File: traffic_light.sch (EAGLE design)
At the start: 58 parts, among them IC1 74LS48N, IC2 74LS48N, IC3 NE555N, IC4 74LS48N, IC5 74LS48N, IC6 74190N, IC7 74190N

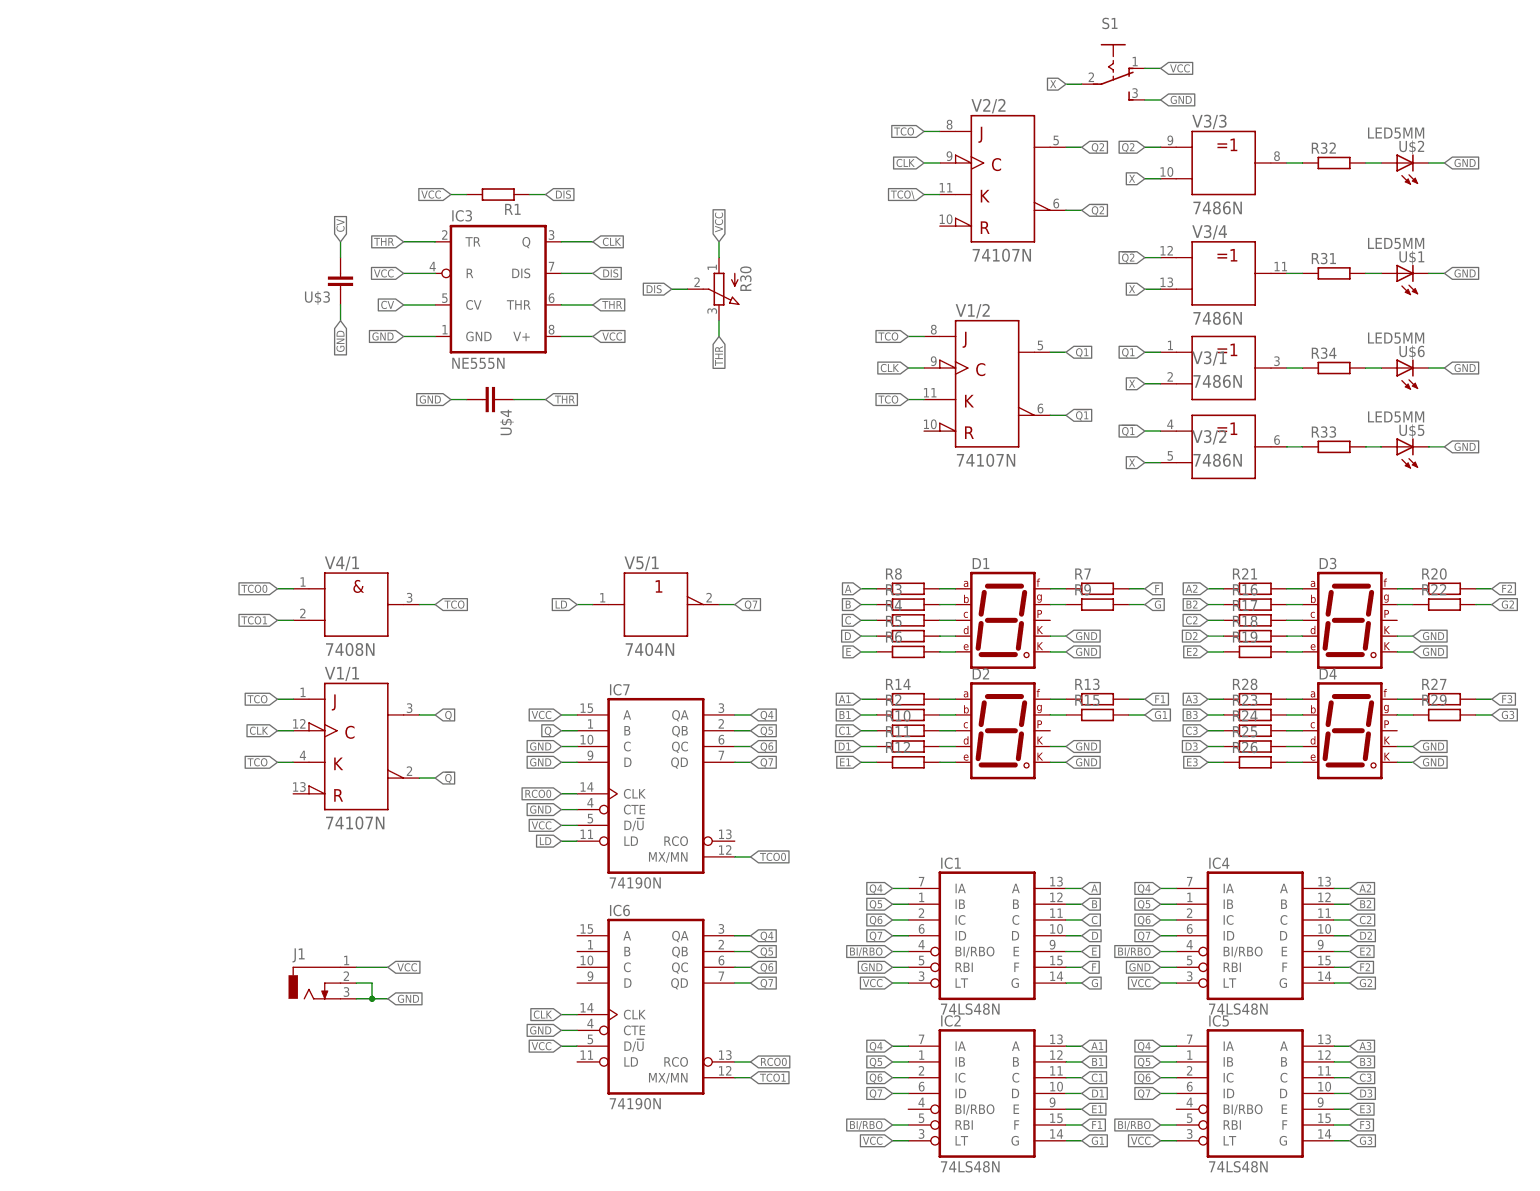
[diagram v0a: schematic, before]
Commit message: commit
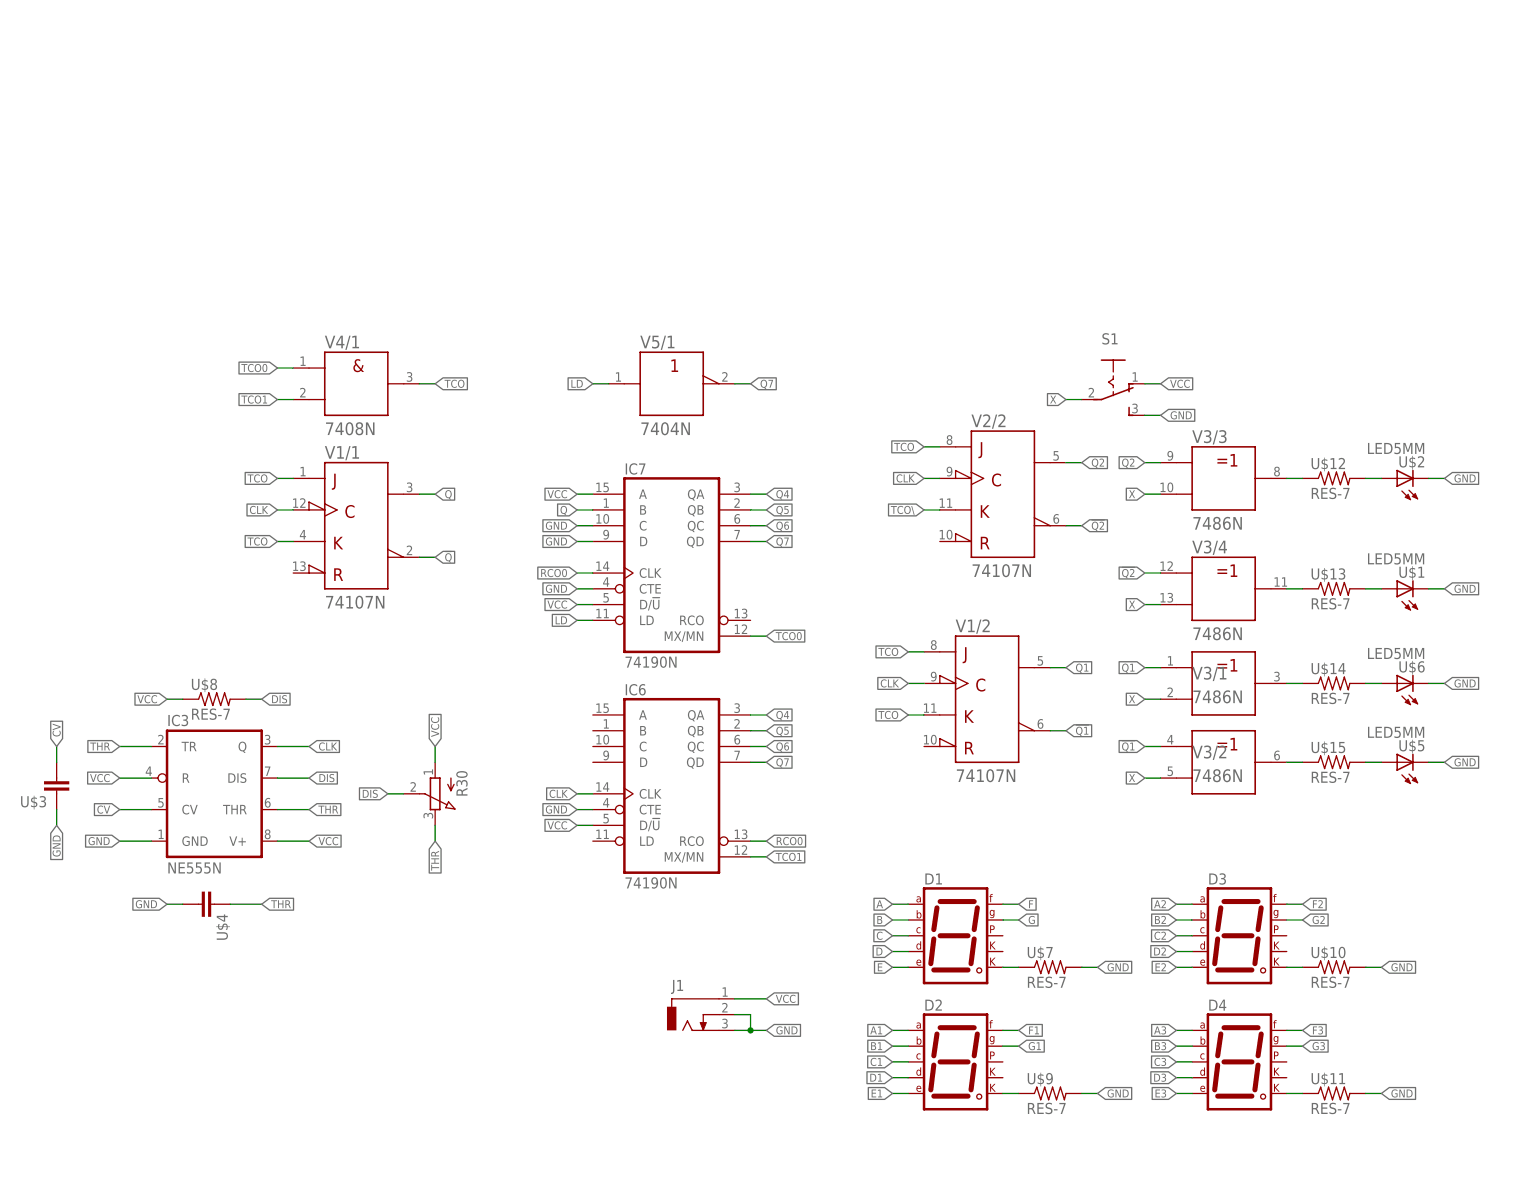
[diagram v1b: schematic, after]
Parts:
- removed IC1, IC2, IC4, IC5: 74LS48N, 74xx-eu:74LS48N
- removed R1, R10, R11, R12, R13, R14, R15, R16, R17, R18, R19, R2, R20, R21, R22, R23, R24, R25, R26, R27, R28, R29, R3, R31, R32, R33, R34, R4, R5, R6, R7, R8, R9: (no value), rcl:R-EU_0207/10
- added U$10, U$11, U$12, U$13, U$14, U$15, U$7, U$8, U$9: RES-7, MIA_LIBRARY-2-2-2:RES-7
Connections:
- removed net BI/RBO: IC1A.BI/RBO, IC2A.RBI, IC4A.BI/RBO, IC5A.RBI
- removed net N$10: D2.D, R11.2
- removed net N$11: D2.E, R12.2
- removed net N$12: D2.F, R13.1
- removed net N$13: D2.G, R15.1
- removed net N$14: D3.B, R16.2
- removed net N$15: D3.C, R17.2
- removed net N$16: D3.D, R18.2
- removed net N$17: D3.E, R19.2
- removed net N$18: D3.F, R20.1
- removed net N$19: D3.G, R22.1
- removed net N$20: D4.B, R23.2
- removed net N$21: D4.C, R24.2
- removed net N$22: D4.D, R25.2
- removed net N$23: D4.E, R26.2
- removed net N$24: D4.F, R27.1
- removed net N$25: D4.G, R29.1
- removed net N$5: D1.E, R6.2
- removed net N$6: D1.F, R7.1
- removed net N$7: D1.G, R9.1
- removed net N$8: D2.B, R2.2
- removed net N$9: D2.C, R10.2
- new net N$1: D1.CK2, U$7.1
- net A: no longer D2.A, D3.A, D4.A, IC1A.A, R14.2, R21.2, R28.2, R8.1, R8.2
- net A1: now also D2.A; no longer IC2A.A, R14.1
- net A2: now also D3.A; no longer IC4A.A, R21.1
- net A3: now also D4.A; no longer IC5A.A, R28.1
- net B: now also D1.B; no longer IC1A.B, R3.1
- net B1: now also D2.B; no longer IC2A.B, R2.1
- net B2: now also D3.B; no longer IC4A.B, R16.1
- net B3: now also D4.B; no longer IC5A.B, R23.1
- net C: now also D1.C; no longer IC1A.C, R4.1
- net C1: now also D2.C; no longer IC2A.C, R10.1
- net C2: now also D3.C; no longer IC4A.C, R17.1
- net C3: now also D4.C; no longer IC5A.C, R24.1
- net D: now also D1.D; no longer IC1A.D, R5.1
- net D1: now also D2.D; no longer IC2A.D, R11.1
- net D2: now also D3.D; no longer IC4A.D, R18.1
- net D3: now also D4.D; no longer IC5A.D, R25.1
- net DIS: now also U$8.2; no longer R1.1
- net E: now also D1.E; no longer IC1A.E, R6.1
- net E1: now also D2.E; no longer IC2A.E, R12.1
- net E2: now also D3.E; no longer IC4A.E, R19.1
- net E3: now also D4.E; no longer IC5A.E, R26.1
- net F: now also D1.F; no longer IC1A.F, R7.2
- net F1: now also D2.F; no longer IC2A.F, R13.2
- net F2: now also D3.F; no longer IC4A.F, R20.2
- net F3: now also D4.F; no longer IC5A.F, R27.2
- net G: now also D1.G; no longer IC1A.G, R9.2
- net G1: now also D2.G; no longer IC2A.G, R15.2
- net G2: now also D3.G; no longer IC4A.G, R22.2
- net G3: now also D4.G; no longer IC5A.G, R29.2
- net GND: now also U$10.2, U$11.2, U$7.2, U$9.2; no longer D1.CK1, D1.CK2, D2.CK1, D2.CK2, D3.CK1, D3.CK2, D4.CK1, D4.CK2, IC1A.RBI, IC4A.RBI
- net N$2: now also D2.CK2, U$9.1; no longer D1.B, R3.2
- net N$27: now also U$12.2; no longer R32.2
- net N$28: now also U$12.1; no longer R32.1
- net N$29: now also U$13.2; no longer R31.2
- net N$3: now also D3.CK2, U$10.1; no longer D1.C, R4.2
- net N$30: now also U$13.1; no longer R31.1
- net N$31: now also U$14.2; no longer R34.2
- net N$32: now also U$14.1; no longer R34.1
- net N$33: now also U$15.2; no longer R33.2
- net N$34: now also U$15.1; no longer R33.1
- net N$4: now also D4.CK2, U$11.1; no longer D1.D, R5.2
- net Q4: no longer IC1A.IA, IC2A.IA, IC4A.IA, IC5A.IA
- net Q5: no longer IC1A.IB, IC2A.IB, IC4A.IB, IC5A.IB
- net Q6: no longer IC1A.IC, IC2A.IC, IC4A.IC, IC5A.IC
- net Q7: no longer IC1A.ID, IC2A.ID, IC4A.ID, IC5A.ID
- net VCC: now also U$8.1; no longer IC1A.LT, IC2A.LT, IC4A.LT, IC5A.LT, R1.2
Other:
- moved on the sheet: D1, D2, D3, D4, IC3, IC6, IC7, J1, R30, S1, U$1, U$2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
